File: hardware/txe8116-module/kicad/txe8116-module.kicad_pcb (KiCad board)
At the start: 2 copper layers, 59.8 x 42.4 mm, 3 parts, among them J1 Screw_Terminal_01x02, U1 TXE8116

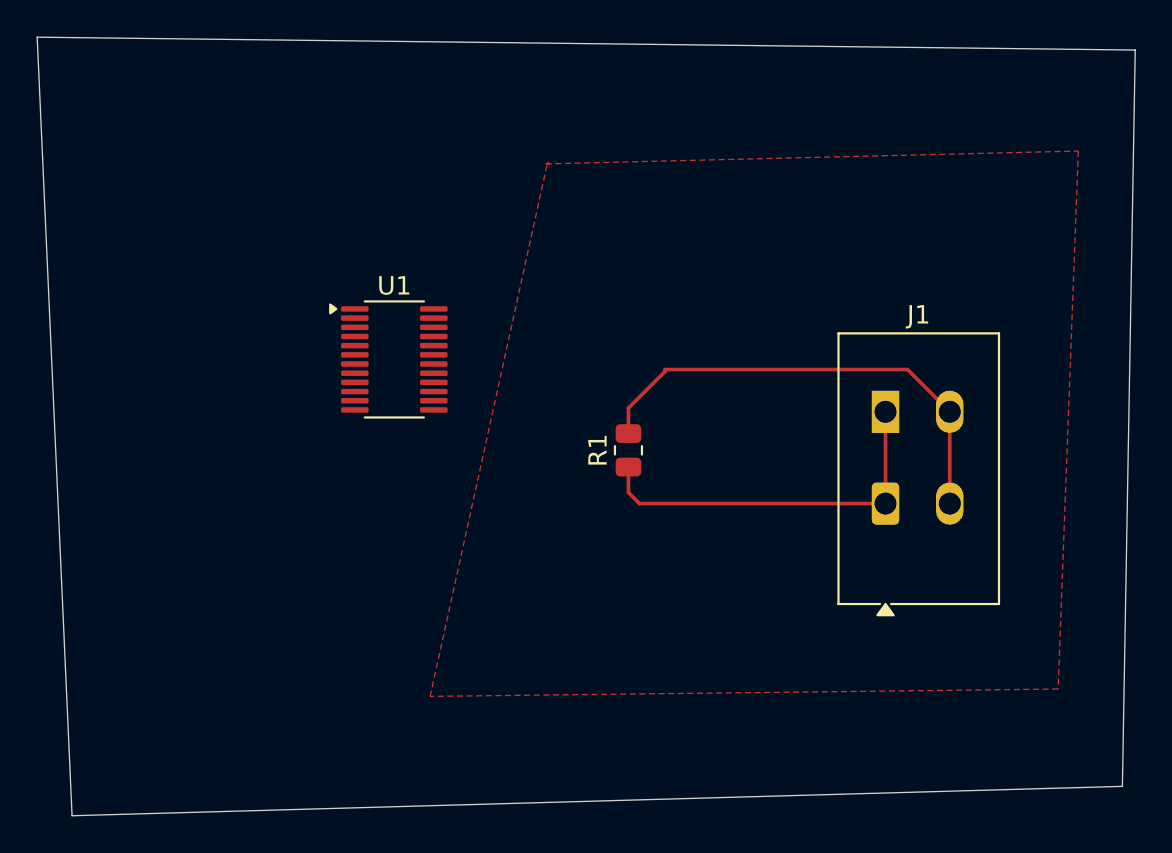
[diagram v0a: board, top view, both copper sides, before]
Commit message: Refactor code structure for improved readability and maintainability
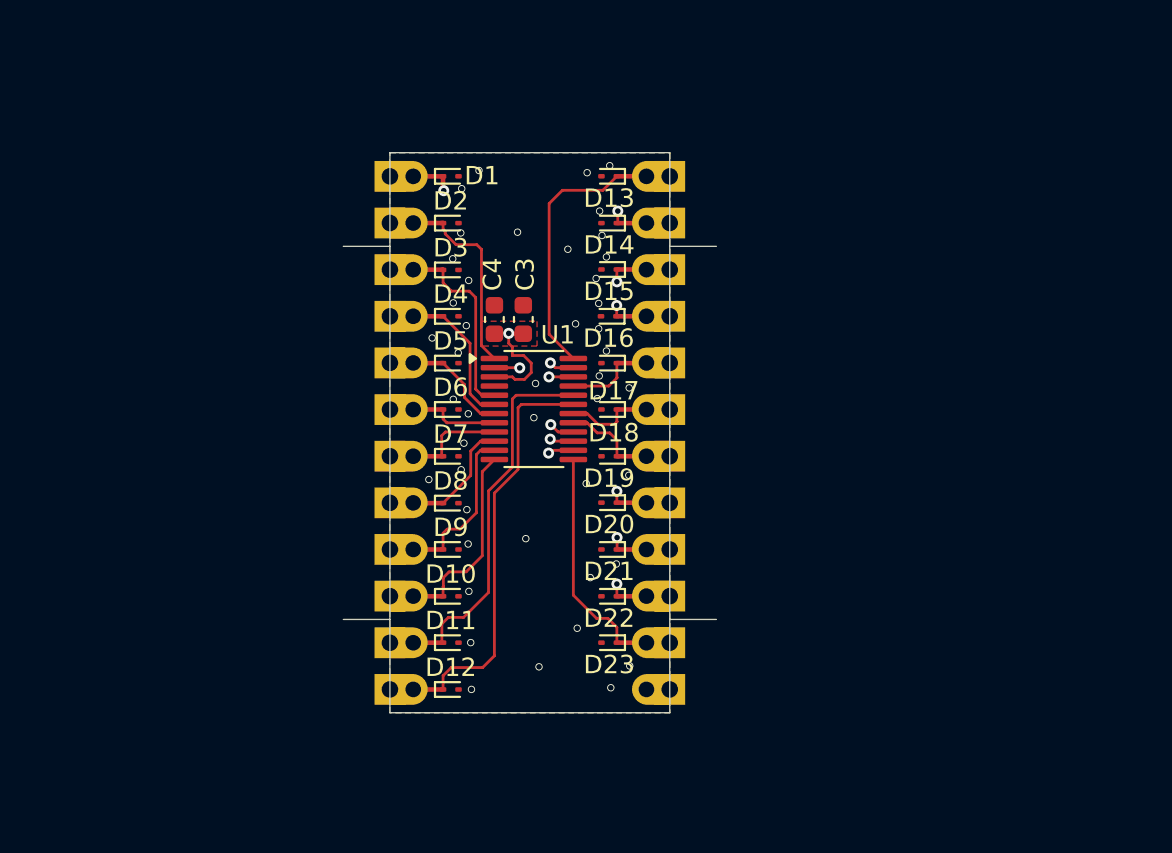
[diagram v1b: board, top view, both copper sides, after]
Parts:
- removed R1: 100k, Resistor_SMD:R_0805_2012Metric
- added C3: 0u1, Capacitor_SMD:C_0603_1608Metric, F.Cu at (150.8, 76.4)
- added C4: 4u7, Capacitor_SMD:C_0603_1608Metric, F.Cu at (149.2, 76.4)
- added D1: ESD9B5.0ST5G, Diode_SMD:D_SOD-923, F.Cu at (146.8, 68.6)
- added D10: ESD9B5.0ST5G, Diode_SMD:D_SOD-923, F.Cu at (146.8, 91.5)
- added D11: ESD9B5.0ST5G, Diode_SMD:D_SOD-923, F.Cu at (146.8, 94.0)
- added D12: ESD9B5.0ST5G, Diode_SMD:D_SOD-923, F.Cu at (146.8, 96.5)
- added D13: ESD9B5.0ST5G, Diode_SMD:D_SOD-923, F.Cu at (155.4, 68.6)
- added D14: ESD9B5.0ST5G, Diode_SMD:D_SOD-923, F.Cu at (155.4, 71.1)
- added D15: ESD9B5.0ST5G, Diode_SMD:D_SOD-923, F.Cu at (155.4, 73.7)
- added D16: ESD9B5.0ST5G, Diode_SMD:D_SOD-923, F.Cu at (155.4, 76.2)
- added D17: ESD9B5.0ST5G, Diode_SMD:D_SOD-923, F.Cu at (155.4, 78.8)
- added D18: ESD9B5.0ST5G, Diode_SMD:D_SOD-923, F.Cu at (155.4, 81.3)
- added D19: ESD9B5.0ST5G, Diode_SMD:D_SOD-923, F.Cu at (155.5, 83.8)
- added D2: ESD9B5.0ST5G, Diode_SMD:D_SOD-923, F.Cu at (146.8, 71.1)
- added D20: ESD9B5.0ST5G, Diode_SMD:D_SOD-923, F.Cu at (155.4, 86.3)
- added D21: ESD9B5.0ST5G, Diode_SMD:D_SOD-923, F.Cu at (155.4, 88.9)
- added D22: ESD9B5.0ST5G, Diode_SMD:D_SOD-923, F.Cu at (155.4, 91.5)
- added D23: ESD9B5.0ST5G, Diode_SMD:D_SOD-923, F.Cu at (155.4, 94.0)
- added D3: ESD9B5.0ST5G, Diode_SMD:D_SOD-923, F.Cu at (146.8, 73.7)
- added D4: ESD9B5.0ST5G, Diode_SMD:D_SOD-923, F.Cu at (146.8, 76.2)
- added D5: ESD9B5.0ST5G, Diode_SMD:D_SOD-923, F.Cu at (146.8, 78.8)
- added D6: ESD9B5.0ST5G, Diode_SMD:D_SOD-923, F.Cu at (146.8, 81.3)
- added D7: ESD9B5.0ST5G, Diode_SMD:D_SOD-923, F.Cu at (146.8, 83.8)
- added D8: ESD9B5.0ST5G, Diode_SMD:D_SOD-923, F.Cu at (146.8, 86.4)
- added D9: ESD9B5.0ST5G, Diode_SMD:D_SOD-923, F.Cu at (146.8, 88.9)
- added J2: Conn_01x12, misc:1x12_P2.54mm_Castellated, F.Cu at (157.5, 68.6)
- J1: value Screw_Terminal_01x02 -> Conn_01x12; footprint TerminalBlock_WAGO:TerminalBlock_WAGO_2601-1102_1x02_P3.50mm_Horizontal -> misc:1x12_P2.54mm_Castellated_Mirrored
- moved J1 31.3 mm to (144.8, 68.6), turned to -90 degrees
- moved U1 8.07 mm to (151.3, 81.2)
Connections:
- J1 pad 1: Net-(J1-Pin_1) -> VCC
- J1 pad 2: Net-(J1-Pin_2) -> /~{INT}
- U1 pad 1: unconnected-(U1-~{INT}-Pad1) -> /~{INT}
- U1 pad 10: unconnected-(U1-P0.5-Pad10) -> /GPIO0.5
- U1 pad 11: unconnected-(U1-P0.6-Pad11) -> /GPIO0.6
- U1 pad 12: unconnected-(U1-P0.7-Pad12) -> /GPIO0.7
- U1 pad 13: unconnected-(U1-P1.7-Pad13) -> /GPIO1.7
- U1 pad 14: unconnected-(U1-P1.6-Pad14) -> /GPIO1.6
- U1 pad 15: unconnected-(U1-P1.5-Pad15) -> /GPIO1.5
- U1 pad 16: unconnected-(U1-P1.4-Pad16) -> /GPIO1.4
- U1 pad 17: unconnected-(U1-P1.3-Pad17) -> /GPIO1.3
- U1 pad 18: unconnected-(U1-P1.2-Pad18) -> /GPIO1.2
- U1 pad 19: unconnected-(U1-P1.1-Pad19) -> /GPIO1.1
- U1 pad 2: unconnected-(U1-SDO-Pad2) -> /SDO
- U1 pad 20: unconnected-(U1-P1.0-Pad20) -> /GPIO1.0
- U1 pad 21: unconnected-(U1-~{CS}-Pad21) -> /~{CS}
- U1 pad 22: unconnected-(U1-SCLK-Pad22) -> /SCLK
- U1 pad 23: unconnected-(U1-SDI-Pad23) -> /SDI
- U1 pad 24: unconnected-(U1-~{RESET}-Pad24) -> /~{RESET}
- U1 pad 3: unconnected-(U1-VCC-Pad3) -> VCC
- U1 pad 4: unconnected-(U1-GND-Pad4) -> GND
- U1 pad 5: unconnected-(U1-P0.0-Pad5) -> /GPIO0.0
- U1 pad 6: unconnected-(U1-P0.1-Pad6) -> /GPIO0.1
- U1 pad 7: unconnected-(U1-P0.2-Pad7) -> /GPIO0.2
- U1 pad 8: unconnected-(U1-P0.3-Pad8) -> /GPIO0.3
- U1 pad 9: unconnected-(U1-P0.4-Pad9) -> /GPIO0.4
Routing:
- net Net-(J1-Pin_2): track 25.8 -> 0.00 mm
- net /GPIO1.1: track 0.00 -> 22.8 mm
- net Net-(J1-Pin_1): track 20.6 -> 0.00 mm
- net /GPIO1.0: track 0.00 -> 20.4 mm
- net VCC: track 0.00 -> 17.7 mm, vias 0 -> 2
- net /SDO: track 0.00 -> 17.1 mm, vias 0 -> 2
- net /~{RESET}: track 0.00 -> 14.9 mm
- net /GPIO1.6: track 0.00 -> 13.1 mm, vias 0 -> 2
- net /GPIO1.7: track 0.00 -> 12.9 mm
- net /SCLK: track 0.00 -> 11.7 mm, vias 0 -> 2
- net /SDI: track 0.00 -> 11.2 mm, vias 0 -> 2
- net /GPIO1.5: track 0.00 -> 11.1 mm, vias 0 -> 2
- net /~{INT}: track 0.00 -> 10.8 mm
- net /GPIO0.7: track 0.00 -> 10.8 mm
- net /GPIO0.0: track 0.00 -> 10.6 mm
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- added copper zone on B.Cu, net GND
- added copper zone on F.Cu, net GND
- added copper zone on In2.Cu, net GND
- added copper zone on F.Cu, net VCC
- removed copper zone on F.Cu, net (none)
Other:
- board size 59.8 x 42.4 mm -> 20.3 x 30.5 mm
- copper layers 2 -> 4
